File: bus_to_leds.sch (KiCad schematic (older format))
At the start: 32 parts

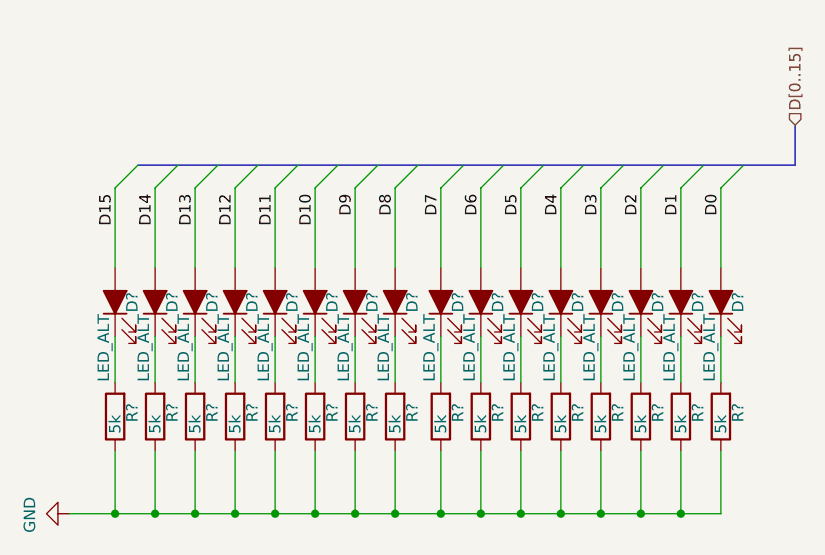
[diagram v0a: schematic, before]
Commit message: way to long since last commit
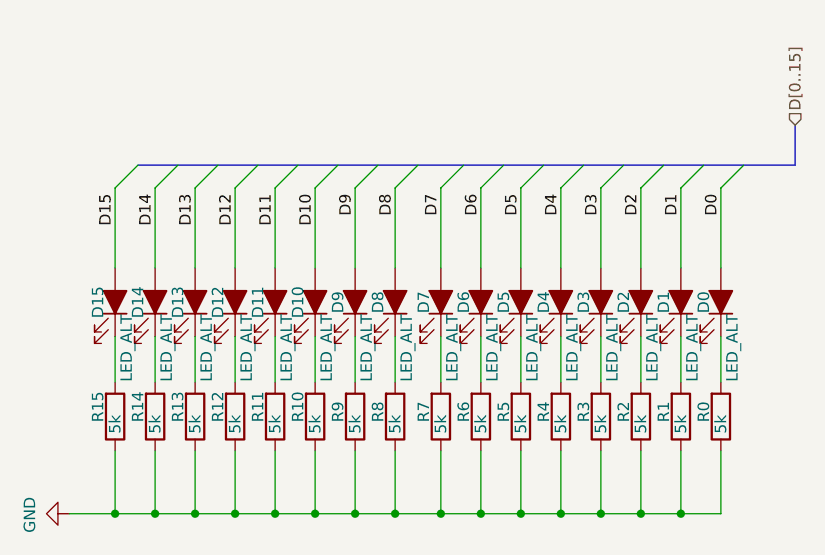
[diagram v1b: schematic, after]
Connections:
- net D0: now also D15.2 (A); no longer D0.2 (A)
- net D1: now also D14.2 (A); no longer D1.2 (A)
- net D10: now also D5.2 (A); no longer D10.2 (A)
- net D11: now also D4.2 (A); no longer D11.2 (A)
- net D12: now also D3.2 (A); no longer D12.2 (A)
- net D13: now also D2.2 (A); no longer D13.2 (A)
- net D14: now also D1.2 (A); no longer D14.2 (A)
- net D15: now also D0.2 (A); no longer D15.2 (A)
- net D2: now also D13.2 (A); no longer D2.2 (A)
- net D3: now also D12.2 (A); no longer D3.2 (A)
- net D4: now also D11.2 (A); no longer D4.2 (A)
- net D5: now also D10.2 (A); no longer D5.2 (A)
- net D6: now also D9.2 (A); no longer D6.2 (A)
- net D7: now also D8.2 (A); no longer D7.2 (A)
- net D8: now also D7.2 (A); no longer D8.2 (A)
- net D9: now also D6.2 (A); no longer D9.2 (A)
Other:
- moved on the sheet: D0, D1, D10, D11, D12, D13, D14, D15, D2, D3, D4, D5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
